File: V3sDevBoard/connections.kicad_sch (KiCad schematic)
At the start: 47 parts, among them J1 JST_ETHERNET, J2 USB_C_Receptacle_USB2.0_16P, J3 USB_C_Receptacle_USB2.0_16P, J4 Micro_SD_Card_Det1, J5 LCD, J6 MIPI CSI, J7 JST_I2C, U12 USBLC6-2SC6, U13 USBLC6-2SC6, U14 USBLC6-2SC6, U15 USBLC6-2SC6, U5 CH340C

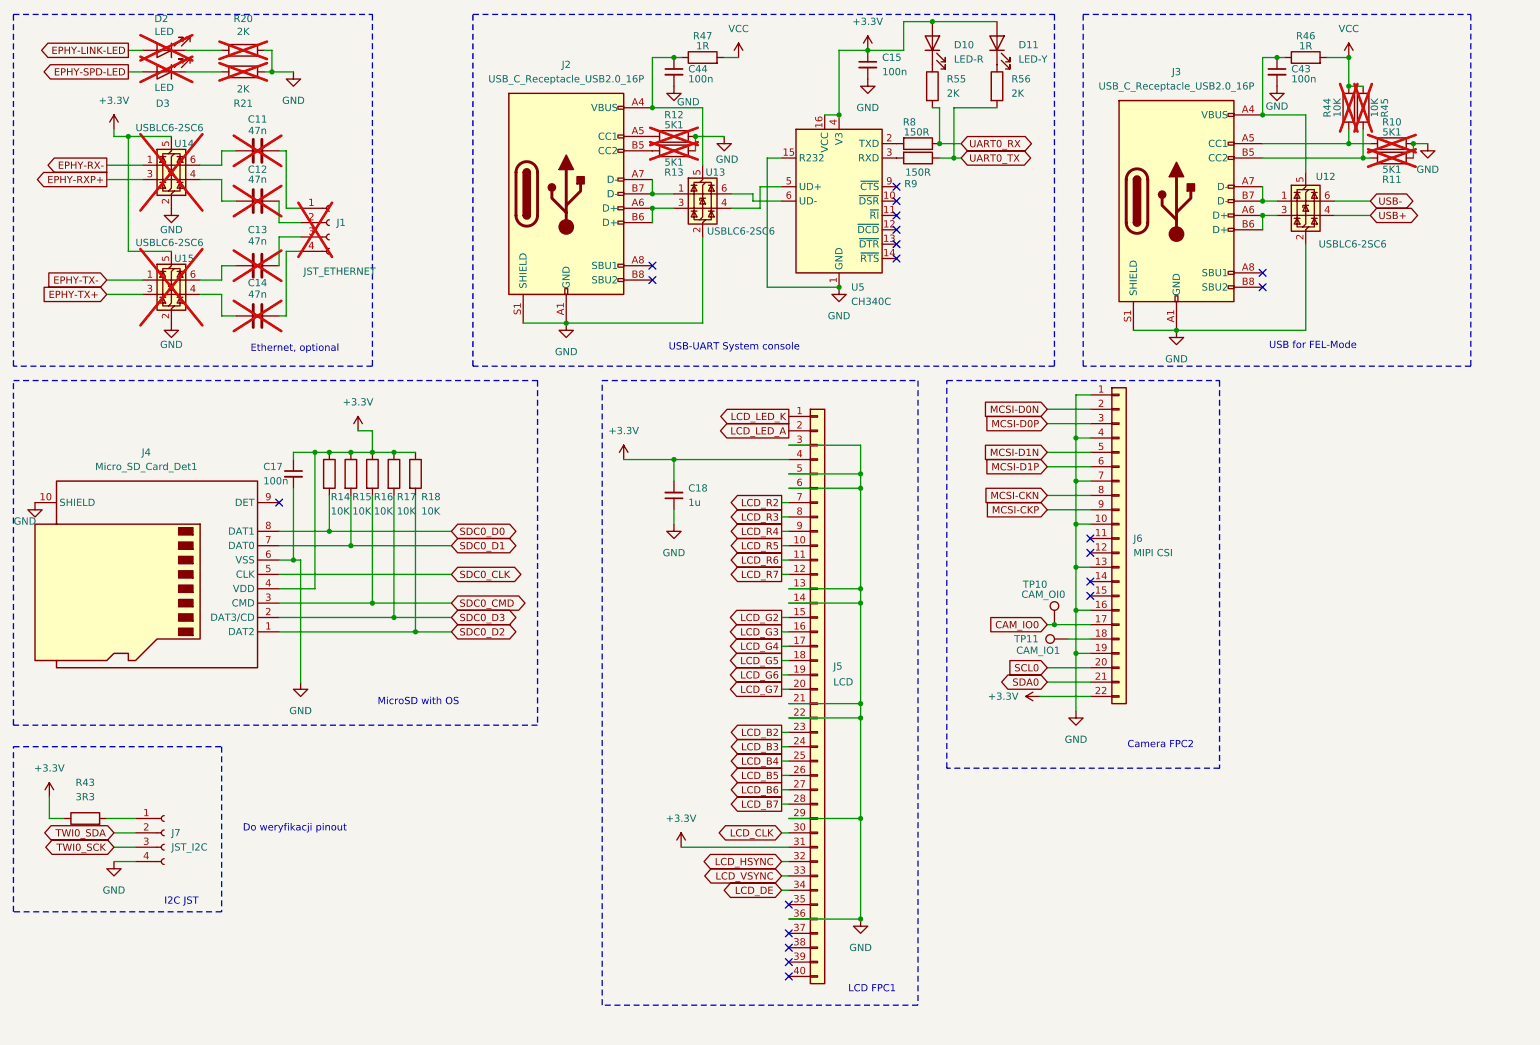
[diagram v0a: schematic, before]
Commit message: completing schematics
completing schematics, adding netclasses, fixing bugs, updating readme, starting pcb
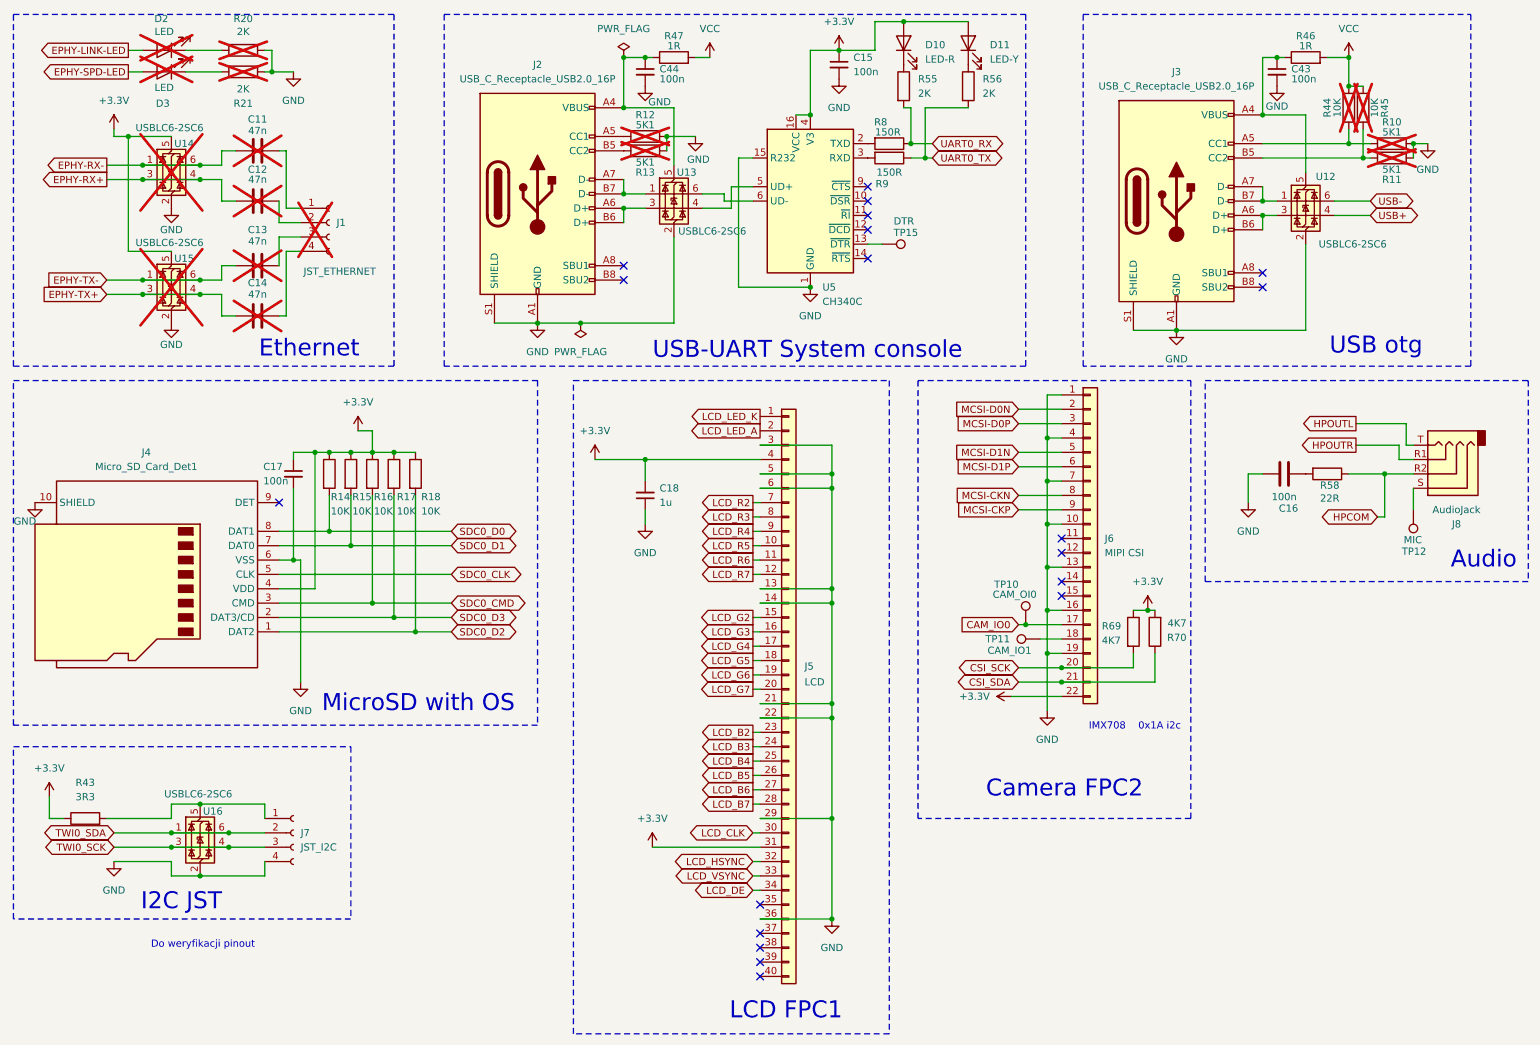
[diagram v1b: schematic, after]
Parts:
- added C16: 100n, Capacitor_SMD:C_0805_2012Metric_Pad1.18x1.45mm_HandSolder, symbol Device:C
- added J8: AudioJack, Connector_Audio:Jack_3.5mm_PJ320D_Horizontal, symbol Connector_Audio:AudioJack4
- added R58: 22R, Resistor_SMD:R_0805_2012Metric_Pad1.20x1.40mm_HandSolder, symbol Device:R
- added R69, R70: 4K7, Resistor_SMD:R_0805_2012Metric_Pad1.20x1.40mm_HandSolder, symbol Device:R
- added TP12: MIC, TestPoint:TestPoint_Pad_D1.0mm, symbol Connector:TestPoint
- added TP15: DTR, TestPoint:TestPoint_Pad_D1.0mm, symbol Connector:TestPoint
- added U16: USBLC6-2SC6, Package_TO_SOT_SMD:SOT-23-6, symbol Power_Protection:USBLC6-2SC6
- C17, C18: footprint (none) -> Capacitor_SMD:C_0805_2012Metric_Pad1.18x1.45mm_HandSolder
- R43: footprint (none) -> Resistor_SMD:R_0805_2012Metric_Pad1.20x1.40mm_HandSolder
- R46, R47: footprint Resistor_SMD:R_0805_2012Metric_Pad1.20x1.40mm_HandSolder -> Resistor_SMD:R_1206_3216Metric
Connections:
- net EPHY-RXP+ is gone; now on net EPHY-RX+: U14.3 (I/O2)
- net +3.3V: now also R69.1, R70.2
- net EPHY-RX-: now also C11.1, U14.6 (I/O1)
- net EPHY-TX+: now also C14.1, U15.4 (I/O2)
- net EPHY-TX-: now also C13.1, U15.6 (I/O1)
- net GND: now also C16.2, U16.2 (GND)
- net TWI0_SCK: now also U16.3 (I/O2), U16.4 (I/O2)
- net TWI0_SDA: now also U16.1 (I/O1), U16.6 (I/O1)
- net at J7.1 (Pin_1), R43.2: now also U16.5 (VBUS)
- net EPHY-RX+: now reaches C12.1, U14.4 (I/O2)
- net at U5.13 (~{DTR}): now also TP15.1
- net SCL0 renamed CSI_SCK
- net CSI_SCK: now also R69.2
- net SDA0 renamed CSI_SDA
- net CSI_SDA: now also R70.1
- new net: J8.S, TP12.1
- new net: C16.1, R58.2
- new net HPCOM: J8.R2, R58.1
- new net HPOUTL: J8.T
- new net HPOUTR: J8.R1
- no-connect marks 20 -> 19
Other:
- note added: "Audio"
- note added: "Ethernet"
- note added: "IMX708 0x1A i2c"
- note added: "USB otg"
- note removed: "Ethernet, optional"
- note removed: "USB for FEL-Mode"
- company: J.K. -> jakub.kmiecik@protonmail.com
- moved on the sheet: C15, C18, C44, D10, D11, J2, J5, J6, J7, R12, R13, R47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
